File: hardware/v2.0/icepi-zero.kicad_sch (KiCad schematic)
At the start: 30 parts, among them J1 Conn_02x20_Counter_Clockwise, SW1 SW_Push, SW2 SW_Push, U1 ECP5U-25F-CABGA256, Y1 SG-8018CG 50.000000MHz

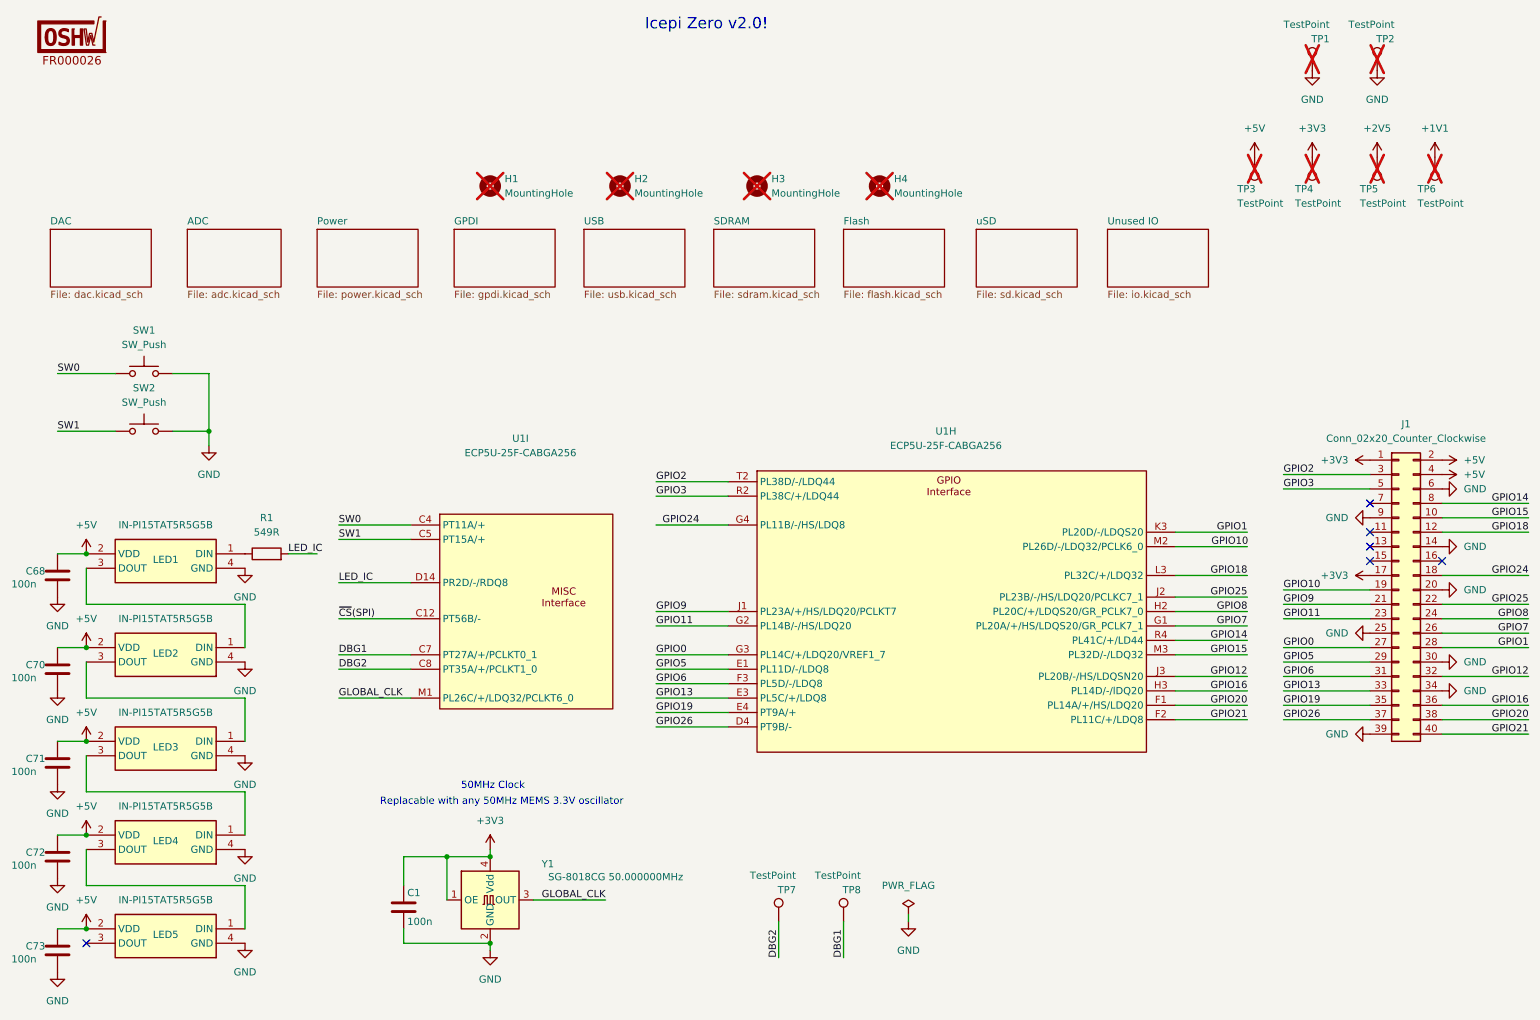
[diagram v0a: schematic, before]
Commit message: DAC Vout
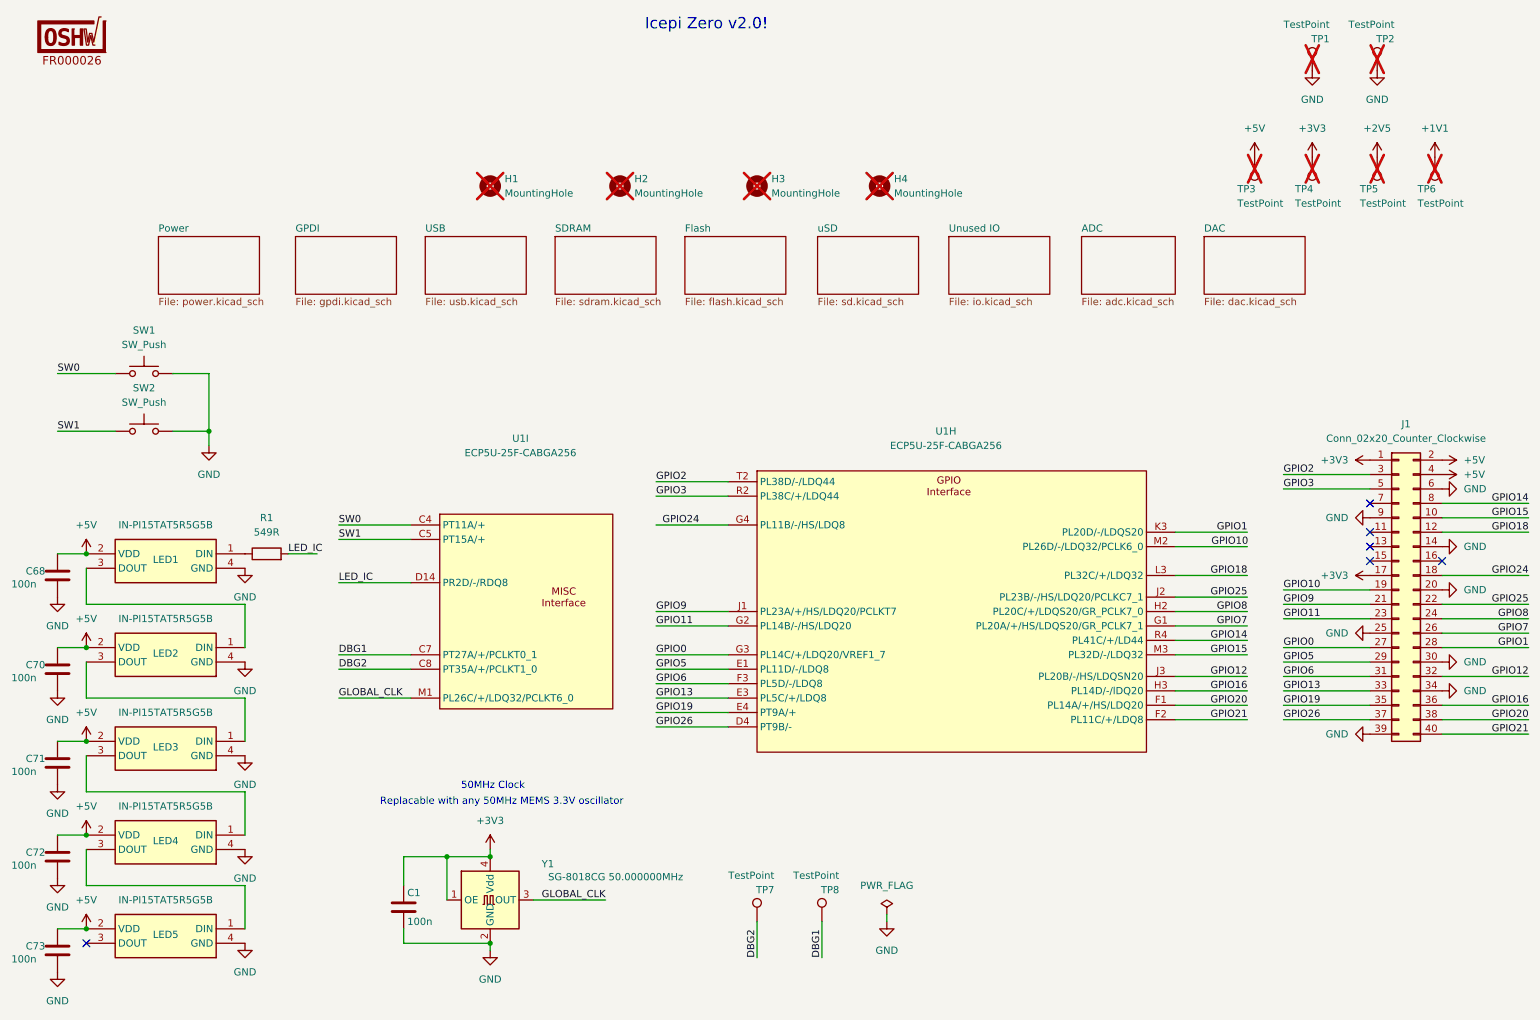
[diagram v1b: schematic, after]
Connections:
- removed net ~{CS}(SPI): U1.C12 (PT56B/-)
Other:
- moved on the sheet: TP7, TP8
